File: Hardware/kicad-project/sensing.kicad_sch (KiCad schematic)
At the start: 34 parts, among them U1 LM358P, U2 LEM-CAS-6NP, U3 LM358P, U4 LM358P

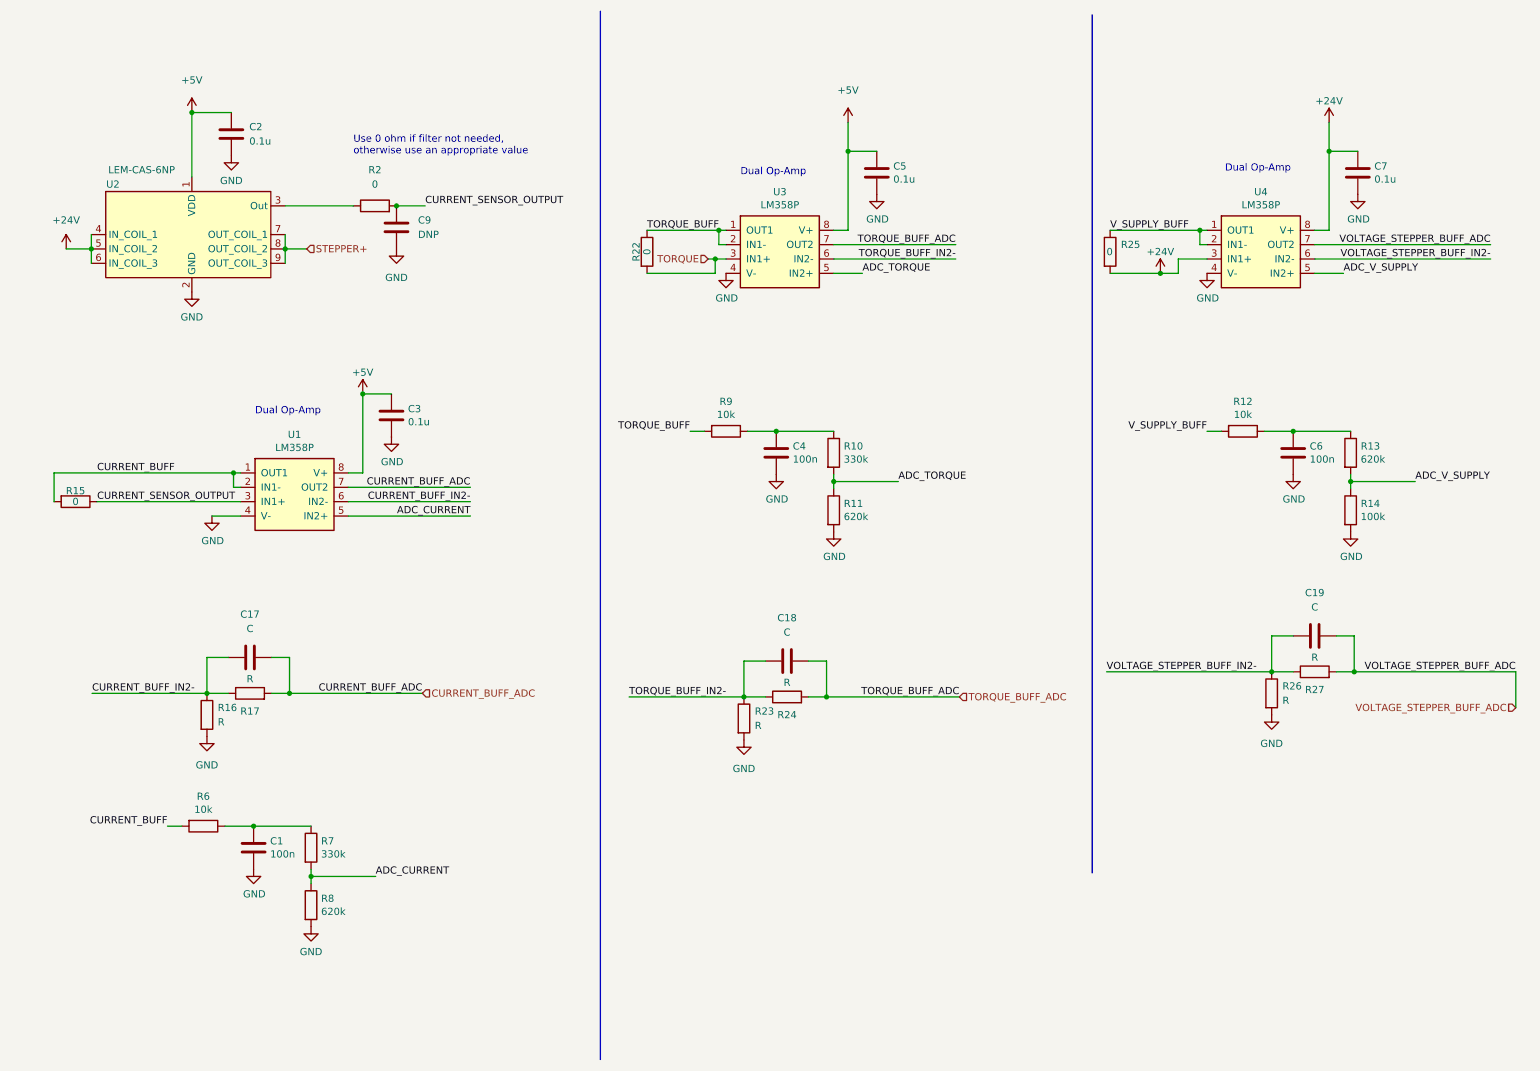
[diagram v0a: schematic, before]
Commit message: hw: update schematic (printable version)
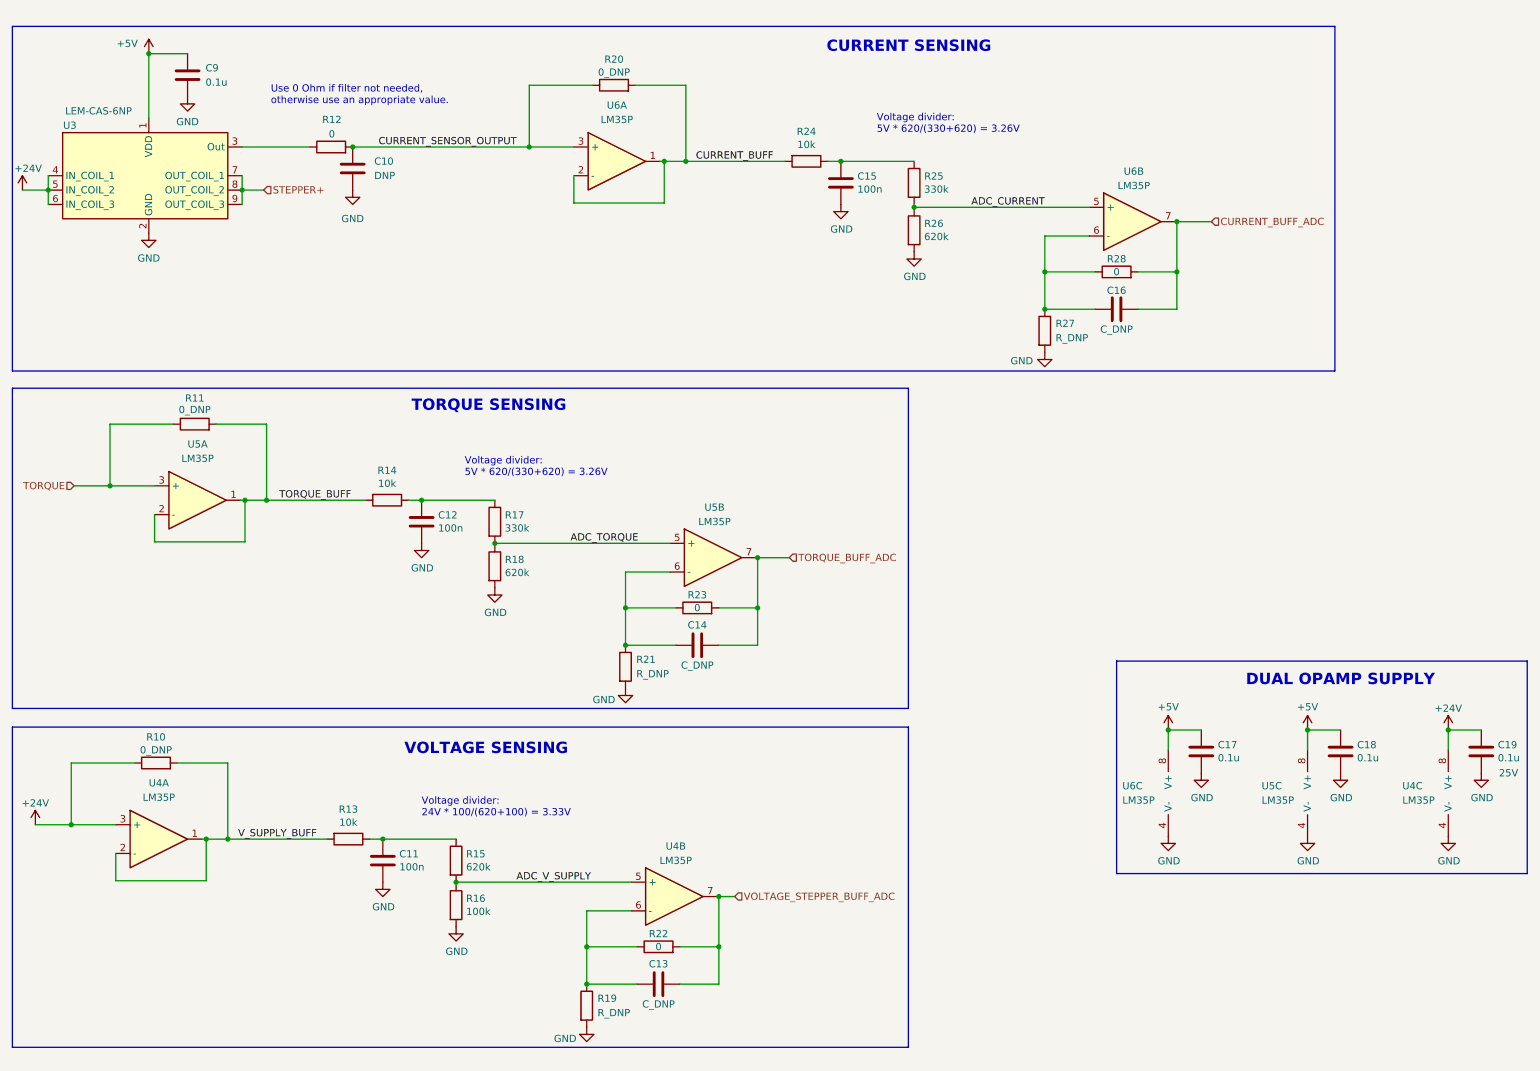
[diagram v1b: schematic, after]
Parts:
- removed C1, C6: 100n, Capacitor_SMD:C_0603_1608Metric, symbol Device:C
- removed C18: C, Capacitor_SMD:C_0805_2012Metric, symbol Device:C
- removed C3, C7: 0.1u, Capacitor_SMD:C_0603_1608Metric, symbol Device:C
- removed R12, R6: 10k, Resistor_SMD:R_0603_1608Metric, symbol Device:R
- removed R14: 100k, Resistor_SMD:R_0603_1608Metric, symbol Device:R
- removed R15: 0, Resistor_SMD:R_0603_1608Metric, symbol Device:R
- removed R17: R, Resistor_SMD:R_0603_1608Metric, symbol Device:R
- removed R7: 330k, Resistor_SMD:R_0603_1608Metric, symbol Device:R
- removed R8: 620k, Resistor_SMD:R_0603_1608Metric, symbol Device:R
- removed U1, U3, U4: LM358P, Package_DIP:DIP-8_W7.62mm, symbol EncoderLib:LM358P
- added C11, C15: 100n, Capacitor_SMD:C_0603_1608Metric, symbol Device:C
- added C13, C14, C16: C_DNP, Capacitor_SMD:C_0805_2012Metric, symbol Device:C
- added R10, R20: 0_DNP, Resistor_SMD:R_0603_1608Metric, symbol Device:R
- added R13: 10k, Resistor_SMD:R_0603_1608Metric, symbol Device:R
- added R19, R21: R_DNP, Resistor_SMD:R_0603_1608Metric, symbol Device:R
- added R22, R28: 0, Resistor_SMD:R_0603_1608Metric, symbol Device:R
- added U4, U5, U6: LM35P, Package_DIP:DIP-8_W7.62mm, symbol Device:Opamp_Dual
- C17: value C -> 0.1u; footprint Capacitor_SMD:C_0805_2012Metric -> Capacitor_SMD:C_0603_1608Metric
- C19: value C -> 0.1u; footprint Capacitor_SMD:C_0805_2012Metric -> Capacitor_SMD:C_0603_1608Metric; V (none) -> 25V
- R11: renamed from R22; value 0 -> 0_DNP
- R16: value R -> 100k
- R23: value R -> 0
- R24: value R -> 10k
- R25: value 0 -> 330k
- R26: value R -> 620k
- R27: value R -> R_DNP
- renumbered C9 to C10, C4 to C12, C5 to C18, C2 to C9, R2 to R12, R9 to R14, R13 to R15, R10 to R17, R11 to R18, U2 to U3
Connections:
- net +24V: now also C19.1, R10.1, U4.3 (+), U4.8 (V+); no longer R25.2
- net +5V: now also C17.1, U5.8 (V+), U6.8 (V+)
- net ADC_CURRENT: now also R25.2, R26.1, U6.5 (+)
- net ADC_TORQUE: now also U5.5 (+)
- net ADC_V_SUPPLY: now also R16.1, U4.5 (+)
- net CURRENT_BUFF: now also R24.2, R20.2, U6.1, U6.2 (-)
- net CURRENT_BUFF_ADC: now also C16.1, R28.2, U6.7; no longer C17.1
- net CURRENT_SENSOR_OUTPUT: now also R20.1, U6.3 (+)
- net GND: now also C17.2, C19.2, R27.2, C11.2, C15.2, R19.2, R21.2, U4.4 (V-), U5.4 (V-), U6.4 (V-); no longer R23.2
- net TORQUE: now also R11.1, U5.3 (+); no longer R11.2
- net TORQUE_BUFF: now also R11.2, U5.1, U5.2 (-); no longer R11.1
- net TORQUE_BUFF_ADC: now also R23.2, C14.1, U5.7; no longer R24.2
- net VOLTAGE_STEPPER_BUFF_ADC: now also C13.1, R22.2, U4.7; no longer C19.1, R27.2
- net V_SUPPLY_BUFF: now also R10.2, R13.2, U4.1, U4.2 (-); no longer R25.1
- net at R15.1: now also C11.1, R13.1
- removed net CURRENT_BUFF_IN2-: C17.2, R16.1
- net TORQUE_BUFF_IN2-: no longer names the net of R23.1
- net TORQUE_BUFF_IN2-: now also C14.2, R21.1, U5.6 (-); no longer R24.1
- removed net VOLTAGE_STEPPER_BUFF_IN2-: C19.2, R26.1, R27.1
- new net: C13.2, R19.1, R22.1, U4.6 (-)
- new net: C16.2, R27.1, R28.1, U6.6 (-)
- new net: C15.1, R24.1, R25.1
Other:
- note added: "CURRENT SENSING"
- note added: "DUAL OPAMP SUPPLY"
- note added: "TORQUE SENSING"
- note added: "Use 0 Ohm if filter not needed, otherwise use an appropriate value."
- note added: "VOLTAGE SENSING"
- note added: "Voltage divider: 24V * 100/(620+100) = 3.33V"
- note added: "Voltage divider: 5V * 620/(330+620) = 3.26V"
- note removed: "Dual Op-Amp"
- note removed: "Use 0 ohm if filter not needed, otherwise use an appropriate value"
- moved on the sheet: C10, C12, C18, C9, R11, R12, R14, R15, R17, R18, U3
